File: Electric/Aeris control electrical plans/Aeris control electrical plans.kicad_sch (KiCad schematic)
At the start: 6 parts, among them J1 Battery barrel jack, J2 Electrical barrel jack, M1 Stepper_Motor_bipolar, U1 Pico, U2 A4988_STEPPER_MOTOR_DRIVER_CA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

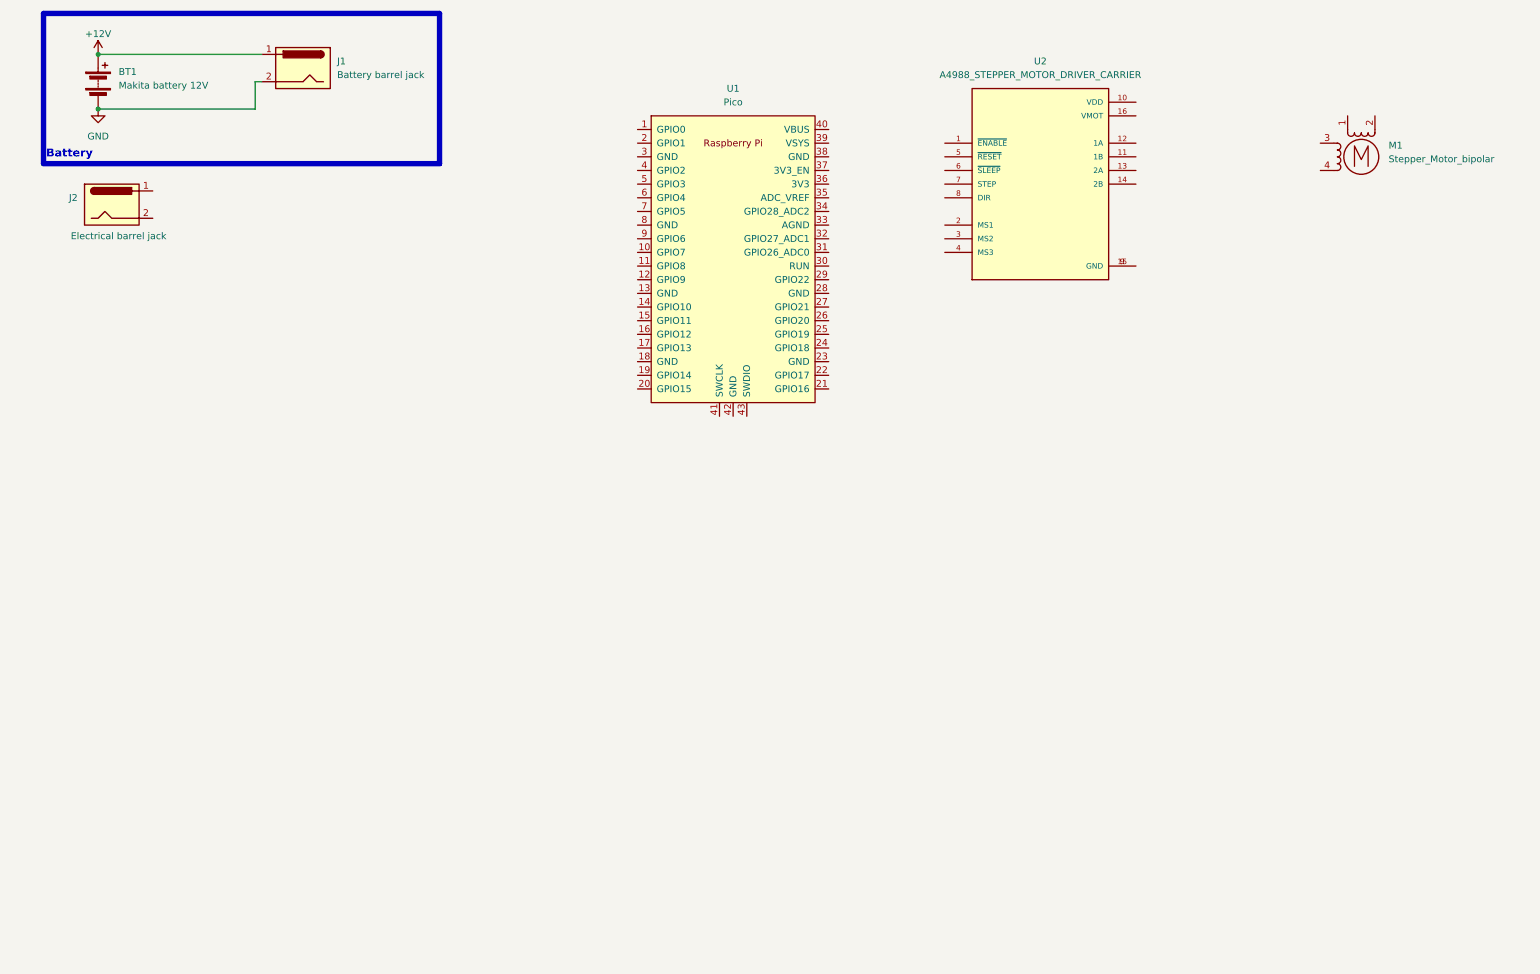
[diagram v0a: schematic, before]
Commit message: push élec presque terminé
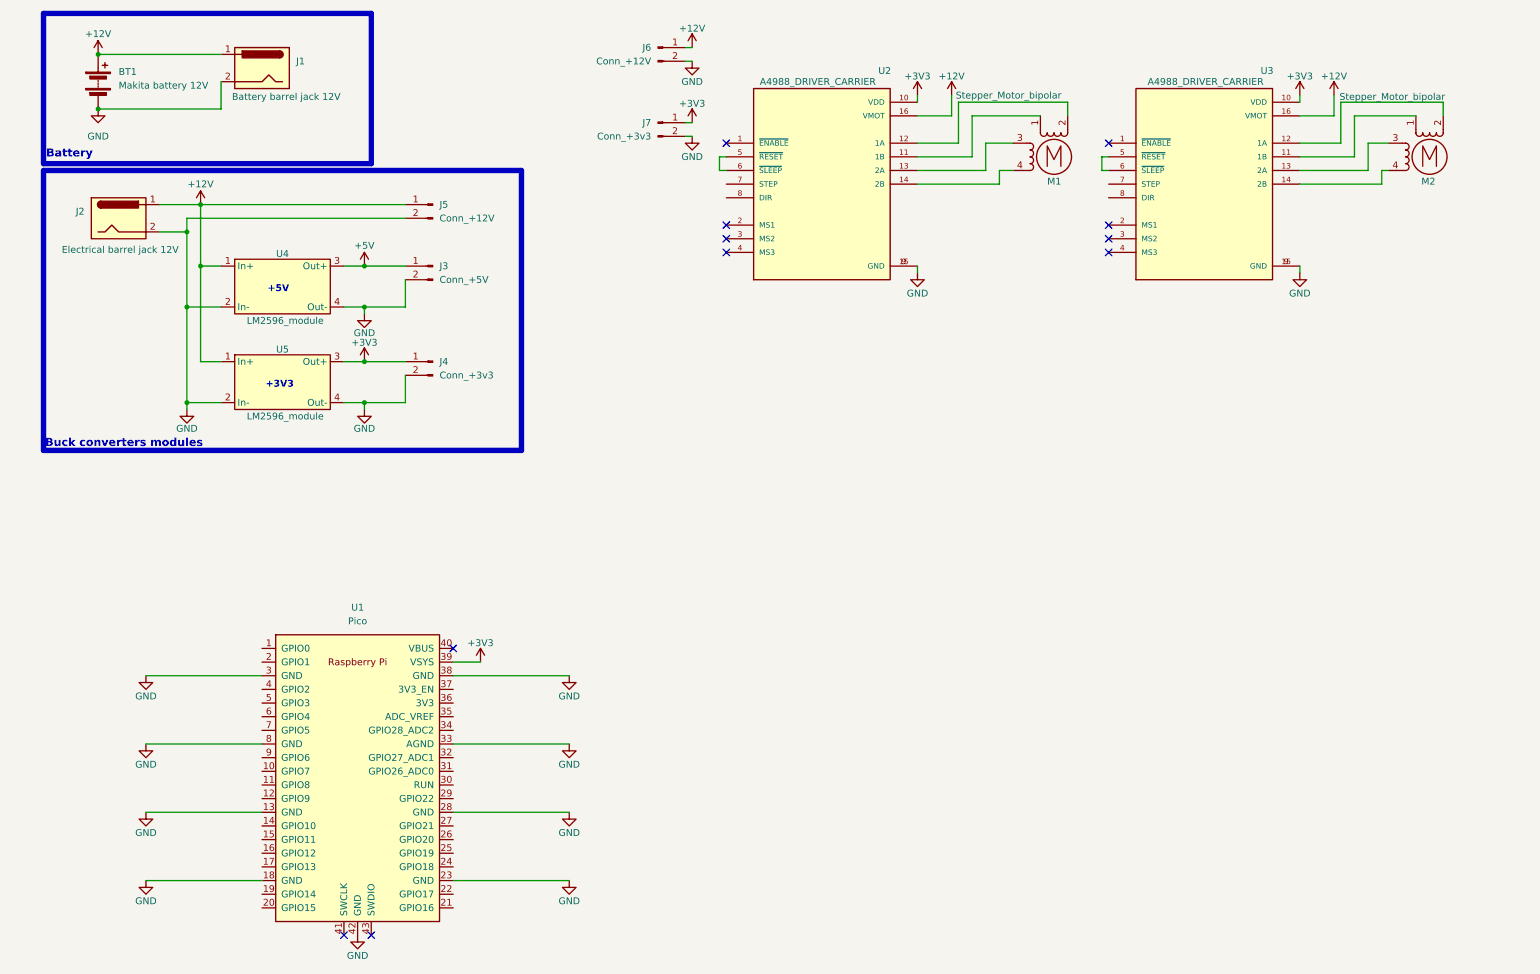
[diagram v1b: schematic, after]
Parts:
- added J3: Conn_+5V, symbol Connector:Conn_01x02_Pin
- added J4, J7: Conn_+3v3, symbol Connector:Conn_01x02_Pin
- added J5, J6: Conn_+12V, symbol Connector:Conn_01x02_Pin
- added M2: Stepper_Motor_bipolar, symbol Motor:Stepper_Motor_bipolar
- added U3: A4988_DRIVER_CARRIER, A4988_STEPPER_MOTOR_DRIVER_CARRIER:MODULE_A4988_STEPPER_MOTOR_DRIVER_CARRIER, symbol A4988:A4988_STEPPER_MOTOR_DRIVER_CARRIER
- added U4, U5: LM2596_module, symbol Buck_converter_modules:LM2596_Module
- J1: value Battery barrel jack -> Battery barrel jack 12V
- J2: value Electrical barrel jack -> Electrical barrel jack 12V
- U2: value A4988_STEPPER_MOTOR_DRIVER_CARRIER -> A4988_DRIVER_CARRIER
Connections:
- net +12V: now also J2.1, U2.16 (VMOT), J5.1 (Pin_1), J6.1 (Pin_1), U3.16 (VMOT), U4.1 (In+), U5.1 (In+)
- net GND: now also J2.2, U1.13 (GND), U1.18 (GND), U1.23 (GND), U1.28 (GND), U1.3 (GND), U1.33 (AGND), U1.38 (GND), U1.42 (GND), U1.8 (GND), U2.15 (GND), U2.9 (GND), J3.2 (Pin_2), J4.2 (Pin_2), J5.2 (Pin_2), J6.2 (Pin_2), J7.2 (Pin_2), U3.15 (GND), U3.9 (GND), U4.2 (In-), U4.4 (Out-), U5.2 (In-), U5.4 (Out-)
- net +3V3: now reaches U2.10 (VDD)
- net +3V3: now also U1.39 (VSYS), J4.1 (Pin_1), J7.1 (Pin_1), U3.10 (VDD), U5.3 (Out+)
- net at U2.11 (1B): now also M1.1
- net at U2.12 (1A): now also M1.2 (-)
- net at U2.13 (2A): now also M1.3
- net at U2.14 (2B): now also M1.4
- net at U2.5 (~{RESET}): now also U2.6 (~{SLEEP})
- new net: M2.1, U3.11 (1B)
- new net: M2.2 (-), U3.12 (1A)
- new net: M2.3, U3.13 (2A)
- new net: M2.4, U3.14 (2B)
- new net: U3.5 (~{RESET}), U3.6 (~{SLEEP})
- new net +5V: J3.1 (Pin_1), U4.3 (Out+)
- no-connect marks 0 -> 11
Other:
- note added: "+3V3"
- note added: "+5V"
- note added: "Buck converters modules"
- moved on the sheet: J1, J2, M1, U1, U2
